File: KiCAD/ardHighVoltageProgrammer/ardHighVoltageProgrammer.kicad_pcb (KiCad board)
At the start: 2 copper layers, 58.4 x 60.3 mm, 8 parts, among them J1 2-pin_power_input_header, Q1 2N3904, U1 ATmega328P-PU, U2 Arduino_Mini_Pro

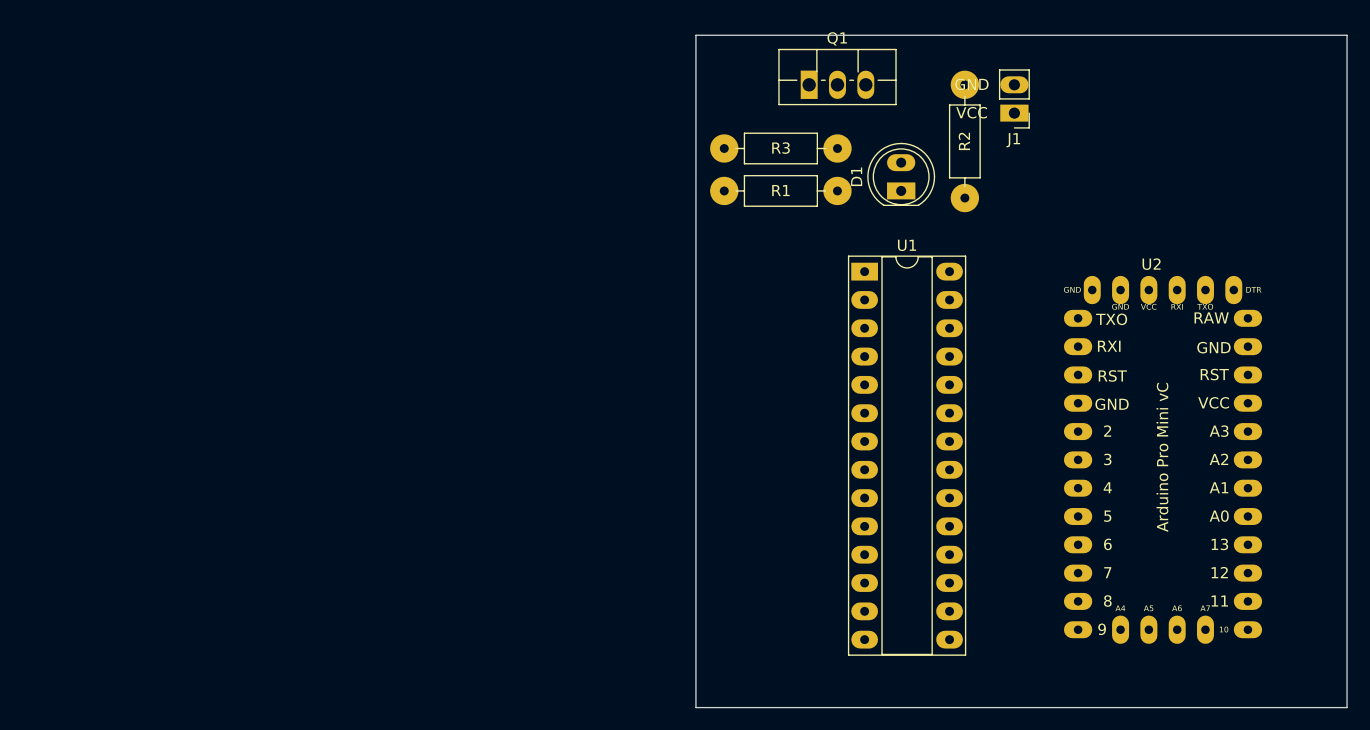
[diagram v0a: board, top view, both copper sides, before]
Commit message: Sketch and cad
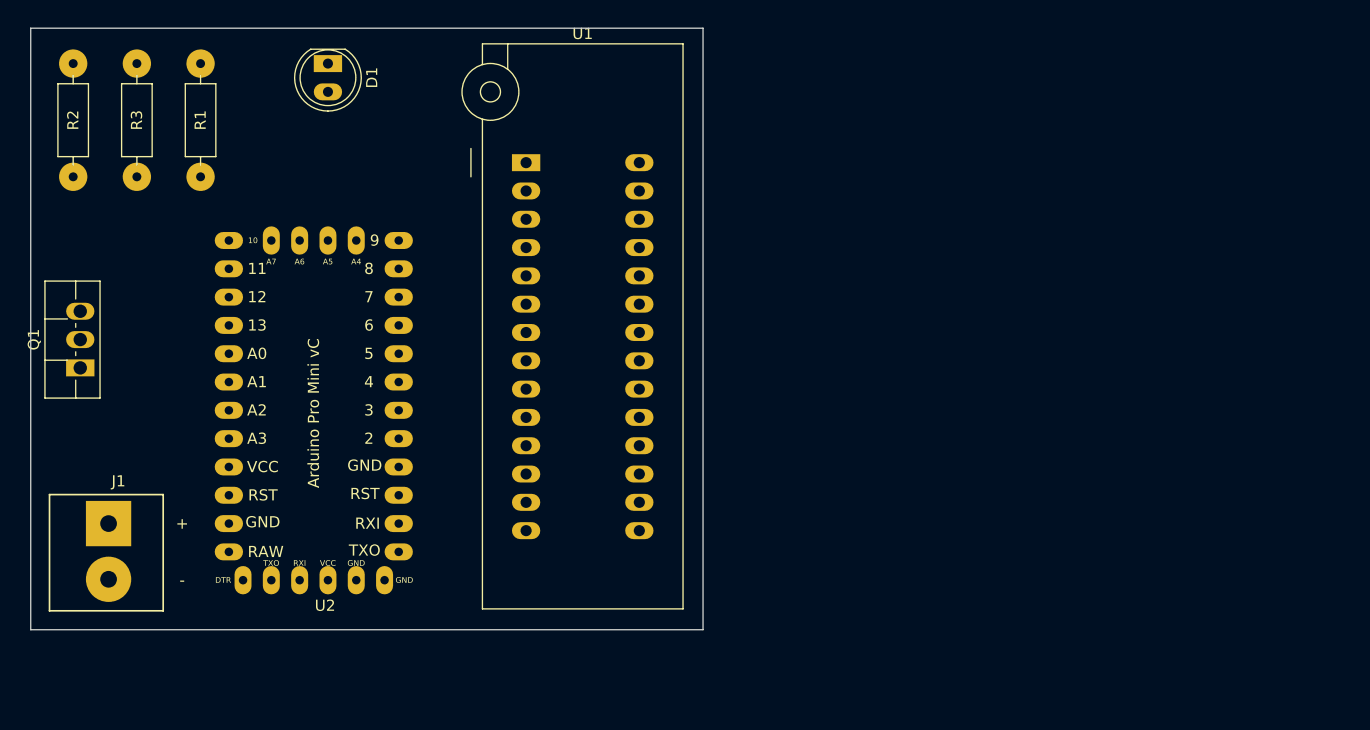
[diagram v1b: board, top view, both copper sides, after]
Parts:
- J1: footprint My_Headers:2-pin_power_input_header_larger_pads -> My_Parts:2-pole_power_in_screw_terminal
- U1: footprint Package_DIP:DIP-28_W7.62mm_Socket_LongPads -> My_Misc:ZIF_DIP_Socket-28_W6.9_W7.62_W10.16_W12.7_W13.5_3M_228-4817-00-0602J_large
- moved J1 89.2 mm to (55.2, 95.9), turned to 0 degrees
- moved R2 80.9 mm to (52.1, 54.6), turned to 270 degrees
- moved Q1 70.2 mm to (52.7, 81.9), turned to 90 degrees
- moved U2 65.1 mm to (82.5, 102.4), turned to 180 degrees
- moved R1 58.3 mm to (63.5, 54.6), turned to 270 degrees
- moved R3 53.3 mm to (57.8, 54.6), turned to 270 degrees
- moved D1 52.7 mm to (74.9, 54.6), turned to 270 degrees
- moved U1 31.9 mm to (92.7, 63.5)
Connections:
- net OE renamed ~OE~
- net RST renamed ~RST~
- net WR renamed ~WR~
- Q1 pad 3: Net-(Q1-Pad3) -> ~RESET~
- R2 pad 2: Net-(Q1-Pad3) -> ~RESET~
- U1 pad 1: RESET -> ~RESET~
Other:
- board size 58.4 x 60.3 mm -> 60.3 x 54 mm
- net class Default: clearance 0.2 -> 0.762; trace_width 0.25 -> 0.508; via_dia 0.8 -> 2.032; via_drill 0.4 -> 0.508
- rule trace_clearance: 0.2 -> 0.762

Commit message: kicad6
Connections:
- net ~OE~ renamed ~{OE}
- net ~RESET~ renamed ~{RESET}
- net ~RST~ renamed ~{RST}
- net ~WR~ renamed ~{WR}
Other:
- net class Default removed
